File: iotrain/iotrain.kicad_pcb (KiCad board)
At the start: 2 copper layers, 24 x 14 mm, 64 parts, among them J1 12V, J10 X2, J11 SCL, J12 SDA, J13 GND, J14 3V3, J15 GND, J2 PROG ESP, J3 AC1, J4 AC1, J5 LSP, J6 LSP, J7 M1, J8 M2, J9 X1, Q1 TPM2008 EP3-A, Q2 TPM2008 EP3-A, SW1 Reset, SW2 Boot, U1 ESP32-C3, U2 MAX98357A_WLP_Package, U3 TPS82130, U6 IPS_160_40_10P, U7 DRV8876RGT, Y1 40MHz

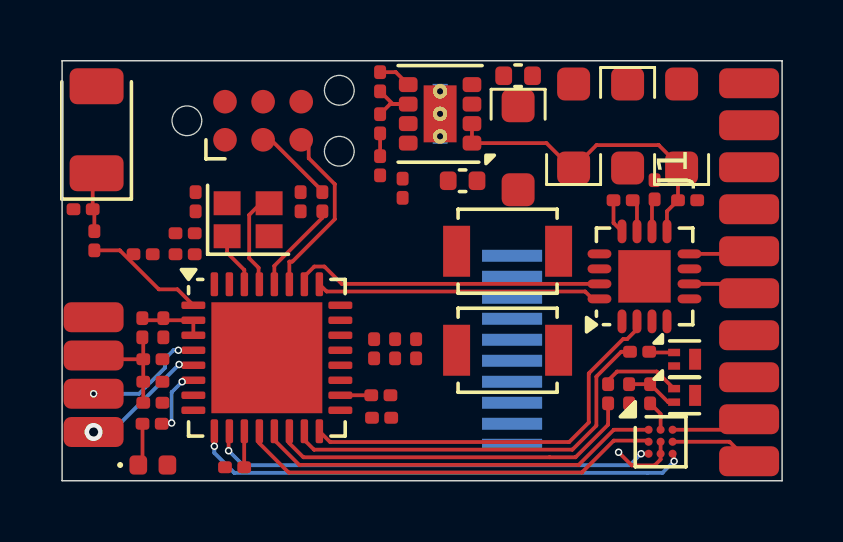
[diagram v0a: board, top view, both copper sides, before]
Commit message: ESP32-C6
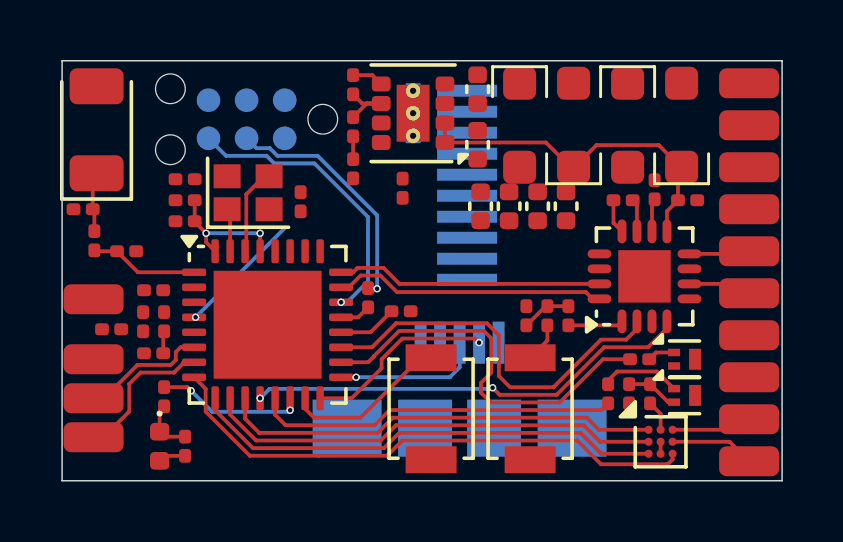
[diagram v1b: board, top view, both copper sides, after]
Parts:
- removed U1: ESP32-C3, Package_DFN_QFN:QFN-32-1EP_5x5mm_P0.5mm_EP3.7x3.7mm
- added C20: 10u/20V, Capacitor_SMD:C_0402_1005Metric, F.Cu at (139.9, 57.5)
- added C22: 10u/20V, Capacitor_SMD:C_0402_1005Metric, F.Cu at (139.0, 57.5)
- added J16: USB_B_Micro, Connector_USB:USB_Micro-B_Amphenol_10104110_Horizontal, B.Cu at (137.3, 63.6)
- added R10: 10k, Resistor_SMD:R_0201_0603Metric, F.Cu at (128.2, 65.5)
- added U4: ESP32-C6FH4, Package_DFN_QFN:QFN-32-1EP_5x5mm_P0.5mm_EP3.6x3.6mm, F.Cu at (130.9, 61.5)
- C11, C13: value 1u -> 10u/20V; footprint Capacitor_SMD:C_0201_0603Metric -> Capacitor_SMD:C_0402_1005Metric
- J2: moved to B.Cu
- L2: value L -> 2n
- moved C11 14.7 mm to (140.9, 57.5), turned to -90 degrees
- moved C13 7.12 mm to (138.1, 57.5), turned to -90 degrees
- moved R8 5.88 mm to (141.0, 61.1)
- moved R7 5.88 mm to (140.3, 61.1)
- moved SW2 5.84 mm to (136.4, 64.2), turned to 90 degrees
- moved U6 5.70 mm to (137.6, 56.8)
- moved C25 4.66 mm to (127.2, 62.4)
- moved C21 3.84 mm to (139.6, 61.1), turned to 90 degrees
- moved C14 3.61 mm to (135.4, 61.0)
- moved R1 3.54 mm to (134.3, 60.5), turned to 90 degrees
- moved C10 2.72 mm to (126.8, 61.4), turned to 90 degrees
- moved C12 2.23 mm to (125.8, 61.6), turned to 180 degrees
- moved SW1 2.09 mm to (139.7, 64.2), turned to 90 degrees
- moved C17 1.42 mm to (137.9, 53.6), turned to -90 degrees
- moved C15 1.30 mm to (137.9, 55.5), turned to -90 degrees
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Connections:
- net Net-(U1-LNA_IN) renamed ANT
- net PROG_IO0 renamed PROG_IO9
- C11 pad 1: +3V3 -> +12V
- C13 pad 1: +3V3 -> +12V
- J2 pad 1: PROG_EN -> CHIP_EN
- R1 pad 1: PROG_TX -> Net-(U4-U0TXD/GPIO16/FSPICS0)
- R1 pad 2: Net-(U1-U0TXD) -> PROG_TX
- R5 pad 1: GND -> unconnected-(R5-Pad1)
- R6 pad 2: Net-(U1-GPIO2) -> INFO_LED
- U6 pad 1: LCD_D -> unconnected-(U6-SDA-Pad1)
- U6 pad 10: GND -> unconnected-(U6-GND-Pad10)
- U6 pad 2: LCD_C -> unconnected-(U6-SCL-Pad2)
- U6 pad 3: LCD_RS -> unconnected-(U6-RS-Pad3)
- U6 pad 4: LCD_RES -> unconnected-(U6-RES-Pad4)
- U6 pad 5: LCD_CS -> unconnected-(U6-CS-Pad5)
- U6 pad 6: GND -> unconnected-(U6-GND-Pad6)
- U6 pad 7: +3V3 -> unconnected-(U6-VCC-Pad7)
- U6 pad 8: +3V3 -> unconnected-(U6-LEDA-Pad8)
- U6 pad 9: LCD_BL -> unconnected-(U6-LEDK-Pad9)
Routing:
- net MOT_IPROPRI: track 0.00 -> 15.0 mm, vias 0 -> 2
- net Net-(J16-D-): track 0.00 -> 6.36 mm, vias 0 -> 1
- net PROG_TX: track 2.47 -> 8.17 mm, vias 0 -> 1
- net PROG_IO9: track 0.00 -> 5.50 mm
- net INFO_LED: track 0.00 -> 4.96 mm, vias 0 -> 2
- net Net-(J16-D+): track 0.00 -> 4.91 mm, vias 0 -> 1
- net CHIP_EN: track 0.00 -> 4.25 mm, vias 0 -> 1
- net PROG_RX: track 5.88 -> 9.73 mm, vias 0 -> 1
- net +3V3: track 8.27 -> 11.9 mm, vias 0 -> 2
- net Net-(U1-U0TXD): track 3.09 -> 0.00 mm
- net Net-(U1-GPIO2): track 2.26 -> 0.00 mm, vias 2 -> 0
- net Net-(C9-Pad1): track 2.23 -> 0.00 mm
- net GND: track 4.00 -> 2.15 mm, vias 1 -> 0
- net PROG_EN: track 0.00 -> 1.66 mm
- net MOT_EN: track 10.5 -> 8.89 mm
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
